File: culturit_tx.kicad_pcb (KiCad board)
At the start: 4 copper layers, 50 x 50 mm, 14 parts, among them J1 USB4105-GF-A, U13 MDBT50Q-1M, U15 BHI260AP

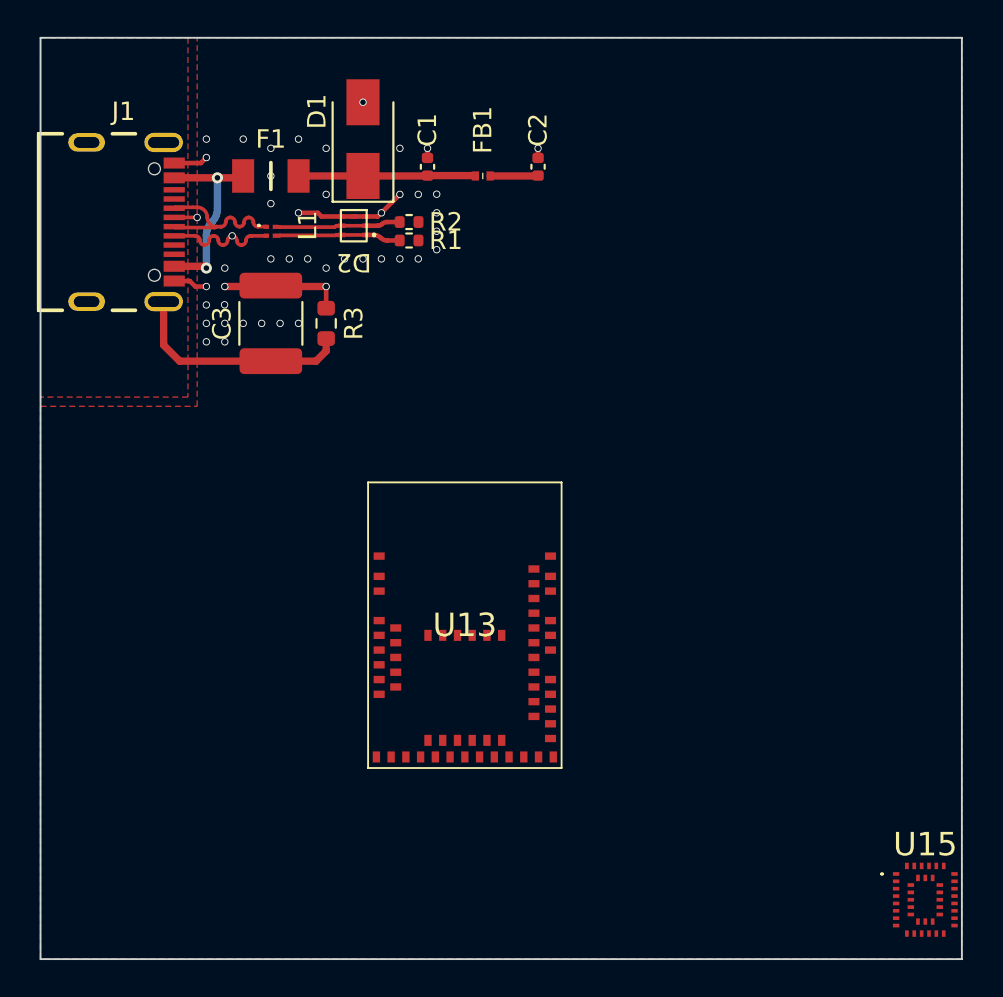
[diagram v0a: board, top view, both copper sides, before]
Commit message: 2022-08-08
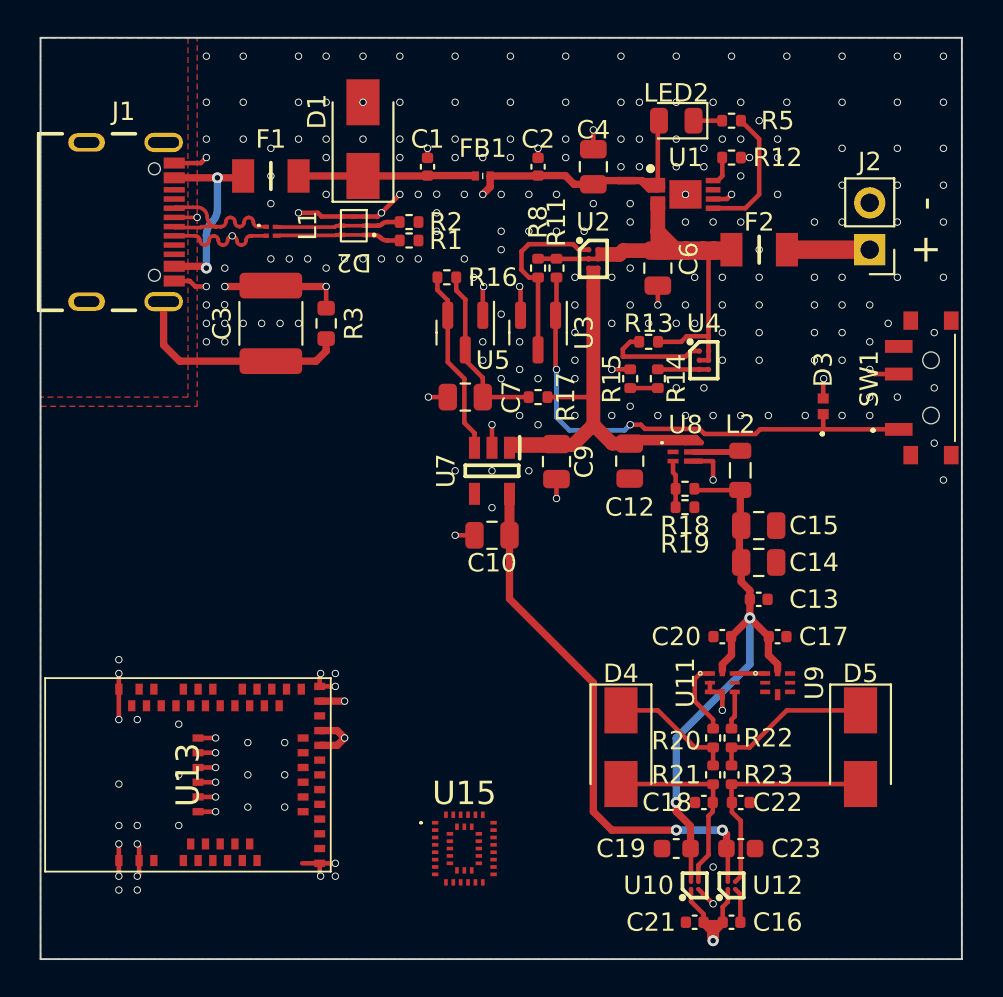
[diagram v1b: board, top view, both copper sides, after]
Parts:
- added C10: 2.2uF(2012), Capacitor_SMD:C_0805_2012Metric, F.Cu at (44.5, 42.0)
- added C12: 4.7uF(2012), Capacitor_SMD:C_0805_2012Metric, F.Cu at (52.0, 38.0)
- added C13: 120pF, Capacitor_SMD:C_0402_1005Metric, F.Cu at (59.0, 45.5)
- added C14: 10uF(2012), Capacitor_SMD:C_0805_2012Metric, F.Cu at (59.0, 43.5)
- added C15: 10uF(2012), Capacitor_SMD:C_0805_2012Metric, F.Cu at (59.0, 41.5)
- added C16: 100nF, Capacitor_SMD:C_0402_1005Metric, F.Cu at (57.5, 63.0)
- added C17: 100nF, Capacitor_SMD:C_0402_1005Metric, F.Cu at (60.0, 47.5)
- added C18: 100nF, Capacitor_SMD:C_0402_1005Metric, F.Cu at (56.0, 56.5)
- added C19: 1uF(1608), Capacitor_SMD:C_0603_1608Metric, F.Cu at (54.5, 59.0)
- added C20: 100nF, Capacitor_SMD:C_0402_1005Metric, F.Cu at (57.0, 47.5)
- added C21: 100nF, Capacitor_SMD:C_0402_1005Metric, F.Cu at (55.5, 63.0)
- added C22: 100nF, Capacitor_SMD:C_0402_1005Metric, F.Cu at (58.0, 56.5)
- added C23: 1uF(1608), Capacitor_SMD:C_0603_1608Metric, F.Cu at (58.0, 59.0)
- added C4: 4.7uF(2012), Capacitor_SMD:C_0805_2012Metric, F.Cu at (50.0, 22.0)
- added C6: 4.7uF(2012), Capacitor_SMD:C_0805_2012Metric, F.Cu at (53.5, 27.5)
- added C7: 2.2uF(2012), Capacitor_SMD:C_0805_2012Metric, F.Cu at (43.0, 34.5)
- added C9: 2.2uF(2012), Capacitor_SMD:C_0805_2012Metric, F.Cu at (48.0, 38.0)
- added D3: LXES1UTAA1-157, Local_devices:LXES1UTAA1157, F.Cu at (62.5, 35.0)
- added D4: SMAJ7.0A, Diode_SMD:D_SMA, F.Cu at (51.5, 53.5)
- added D5: SMAJ7.0A, Diode_SMD:D_SMA, F.Cu at (64.5, 53.5)
- added F2: 0ZCJ0075FF2E, Local_devices:FUSC3216X120N, F.Cu at (59.0, 26.5)
- added J2: Battery, Connector_PinHeader_2.54mm:PinHeader_1x02_P2.54mm_Vertical, F.Cu at (65.0, 26.5)
- added L2: 470nH, Inductor_SMD:L_0805_2012Metric, F.Cu at (58.0, 38.5)
- added LED2: ORANGE, LED_SMD:LED_0805_2012Metric, F.Cu at (54.5, 19.5)
- added R11: 2M, Resistor_SMD:R_0402_1005Metric, F.Cu at (48.0, 27.5)
- added R12: 10k, Resistor_SMD:R_0402_1005Metric, F.Cu at (57.5, 21.5)
- added R13: 1M, Resistor_SMD:R_0402_1005Metric, F.Cu at (53.0, 31.5)
- added R14: 300k, Resistor_SMD:R_0402_1005Metric, F.Cu at (53.5, 33.5)
- added R15: 180k, Resistor_SMD:R_0402_1005Metric, F.Cu at (52.0, 33.5)
- added R16: 0, Resistor_SMD:R_0402_1005Metric, F.Cu at (42.0, 28.0)
- added R17: 1k, Resistor_SMD:R_0402_1005Metric, F.Cu at (47.0, 34.5)
- added R18: 200k, Resistor_SMD:R_0402_1005Metric, F.Cu at (55.0, 39.5)
- added R19: 100k, Resistor_SMD:R_0402_1005Metric, F.Cu at (55.0, 40.5)
- added R20: 100, Resistor_SMD:R_0402_1005Metric, F.Cu at (56.5, 53.0)
- added R21: 1.91k, Resistor_SMD:R_0402_1005Metric, F.Cu at (56.5, 55.0)
- added R22: 100, Resistor_SMD:R_0402_1005Metric, F.Cu at (57.5, 53.0)
- added R23: 1.91k, Resistor_SMD:R_0402_1005Metric, F.Cu at (57.5, 55.0)
- added R5: 470, Resistor_SMD:R_0402_1005Metric, F.Cu at (57.5, 19.5)
- added R8: 1M, Resistor_SMD:R_0402_1005Metric, F.Cu at (47.0, 27.5)
- added SW1: PCM12SMTR, Local_devices:PCM12SMTR, F.Cu at (68.3, 34.0)
- added U1: MCP73832T-2ACI_MC, Local_devices:SON50P300X200X100-9N-D, F.Cu at (55.0, 23.5)
- added U10: TPS22916CNYFPT, Local_devices:BGA4C40P2X2_78X78X50, F.Cu at (55.5, 61.0)
- added U11: SN74AUP2G08RSER, Local_devices:RSE0008A, F.Cu at (57.0, 50.0)
- added U12: TPS22916CNYFPT, Local_devices:BGA4C40P2X2_78X78X50, F.Cu at (57.5, 61.0)
- added U2: CSD25304W1015, Local_devices:BGA6C50P2X3_95X145X62, F.Cu at (50.0, 27.0)
- added U3: DMN65D8L-7, Package_TO_SOT_SMD:SOT-23, F.Cu at (47.0, 31.0)
- added U4: CSD25304W1015, Local_devices:BGA6C50P2X3_95X145X62, F.Cu at (56.0, 32.5)
- added U5: TPS3839A09DBZR, Package_TO_SOT_SMD:SOT-23, F.Cu at (43.0, 31.0)
- added U7: LP5907QMFX-2.8Q1, Local_devices:SOT95P280X145-5N, F.Cu at (44.5, 38.5)
- added U8: TPS6282618DMQR, Local_devices:TPS6282618DMQR, F.Cu at (55.0, 37.5)
- added U9: SN74AUP2G08RSER, Local_devices:RSE0008A, F.Cu at (60.0, 50.0)
- moved U15 25.2 mm to (43.0, 59.0)
- moved U13 17.1 mm to (28.0, 55.0), turned to 90 degrees
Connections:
- U13 pad 1: unconnected-(U13-Pad1) -> Earth
- U13 pad 15: unconnected-(U13-Pad15) -> Earth
- U13 pad 2: unconnected-(U13-Pad2) -> Earth
- U13 pad 28: unconnected-(U13-Pad28) -> +1V8
- U13 pad 30: unconnected-(U13-Pad30) -> +1V8
- U13 pad 32: unconnected-(U13-Pad32) -> VUSB
- U13 pad 33: unconnected-(U13-Pad33) -> Earth
- U13 pad 55: unconnected-(U13-Pad55) -> Earth
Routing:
- net +1V8: track 0.00 -> 62.2 mm, vias 0 -> 3
- net VUSB: track 2.61 -> 50.7 mm, vias 0 -> 2
- net /Power/VDRAIN: track 0.00 -> 47.0 mm
- net +2V8: track 0.00 -> 34.0 mm, vias 0 -> 2
- net Earth: track 17.6 -> 50.0 mm, vias 44 -> 242
- net +BATT: track 0.00 -> 31.0 mm
- net Net-(D3-Pad1): track 0.00 -> 27.8 mm, vias 0 -> 2
- net Net-(C22-Pad1): track 0.00 -> 12.6 mm
- net Net-(C18-Pad1): track 0.00 -> 10.6 mm
- net /Power/UVL_RST: track 0.00 -> 10.1 mm
- net Net-(R8-Pad1): track 0.00 -> 9.94 mm
- net Net-(C7-Pad2): track 0.00 -> 9.64 mm
- net VDD: track 0.00 -> 9.30 mm, vias 0 -> 1
- net Net-(D5-Pad1): track 0.00 -> 8.81 mm
- net Net-(L2-Pad1): track 0.00 -> 7.55 mm
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- added copper zone on In2.Cu, net Earth
- added copper zone on In2.Cu, net VDD
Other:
- board text added: "+"
- board text added: "-"
